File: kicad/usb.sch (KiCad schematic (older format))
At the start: 10 parts, among them J1 USB-C/16p, U2 CH340C, U3 AMS1117-3.3

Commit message: Changelog eingeführt, GND statt GNDD
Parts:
- C1, C2: PriceForQty 500 -> (none)
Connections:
- net labels removed: GNDD
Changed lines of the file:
@@
 F 8 "" H 4100 2400 50  0001 C CNN "PartNr"
 F 9 "0.002141" H 4100 2400 50  0001 C CNN "PriceEUR"
-F 10 "500" H 4100 2400 50  0001 C CNN "PriceForQty"
+F 10 "500
+" H 4100 2400 50  0001 C CNN "PriceForQty"
 F 11 "https://lcsc.com/product-detail/Multilayer-Ceramic-Capacitors-MLCC-SMD-SMT_Walsin-Tech-Corp-0603B104K160CT_C80516.html" H 4100 2400 50  0001 C CNN "Weblink"
 F 12 "C80516" H 4100 2400 50  0001 C CNN "DistOrderNr"
@@
 $EndComp
 $Comp
-L power:GNDD #PWR?
+L power:GND #PWR?
 U 1 1 5F7120DC
 P 4350 2400
@@
 	3350 3000 3400 3000
 $Comp
-L power:GNDD #PWR?
+L power:GND #PWR?
 U 1 1 5F764C96
 P 2900 3000
@@
 F 8 "" H 3400 2400 50  0001 C CNN "PartNr"
 F 9 "0.002141" H 3400 2400 50  0001 C CNN "PriceEUR"
-F 10 "500" H 3400 2400 50  0001 C CNN "PriceForQty"
+F 10 "500
+" H 3400 2400 50  0001 C CNN "PriceForQty"
 F 11 "https://lcsc.com/product-detail/Multilayer-Ceramic-Capacitors-MLCC-SMD-SMT_Walsin-Tech-Corp-0603B104K160CT_C80516.html" H 3400 2400 50  0001 C CNN "Weblink"
 F 12 "C80516" H 3400 2400 50  0001 C CNN "DistOrderNr"
@@
 $EndComp
 $Comp
-L power:GNDD #PWR?
+L power:GND #PWR?
 U 1 1 5F767C48
 P 3150 2400
@@
 $EndComp
 $Comp
-L power:GNDD #PWR?
+L power:GND #PWR?
 U 1 1 60590650
 P 3800 4150
@@
 AR Path="/5F8D661A/60590650" Ref="#PWR012"  Part="1"
 F 0 "#PWR012" H 3800 3900 50  0001 C CNN
-F 1 "GNDD" H 3804 3995 50  0000 C CNN
+F 1 "GND" H 3804 3995 50  0000 C CNN
 F 2 "" H 3800 4150 50  0001 C CNN
 F 3 "" H 3800 4150 50  0001 C CNN
@@
 $EndComp
 $Comp
-L power:GNDD #PWR?
+L power:GND #PWR?
 U 1 1 605914DB
 P 1350 4200
@@
 AR Path="/5F8D661A/605914DB" Ref="#PWR07"  Part="1"
 F 0 "#PWR07" H 1350 3950 50  0001 C CNN
-F 1 "GNDD" H 1354 4045 50  0000 C CNN
+F 1 "GND" H 1354 4045 50  0000 C CNN
 F 2 "" H 1350 4200 50  0001 C CNN
 F 3 "" H 1350 4200 50  0001 C CNN
@@
 $EndComp
 $Comp
-L power:GNDD #PWR?
+L power:GND #PWR?
 U 1 1 60591BD5
 P 1650 4200
@@
 AR Path="/5F8D661A/60591BD5" Ref="#PWR08"  Part="1"
 F 0 "#PWR08" H 1650 3950 50  0001 C CNN
-F 1 "GNDD" H 1654 4045 50  0000 C CNN
+F 1 "GND" H 1654 4045 50  0000 C CNN
 F 2 "" H 1650 4200 50  0001 C CNN
 F 3 "" H 1650 4200 50  0001 C CNN
@@
 $EndComp
 $Comp
-L power:GNDD #PWR?
+L power:GND #PWR?
 U 1 1 605932E8
 P 6300 2350
@@
 AR Path="/5F8D661A/605932E8" Ref="#PWR014"  Part="1"
 F 0 "#PWR014" H 6300 2100 50  0001 C CNN
-F 1 "GNDD" H 6304 2195 50  0000 C CNN
+F 1 "GND" H 6304 2195 50  0000 C CNN
 F 2 "" H 6300 2350 50  0001 C CNN
 F 3 "" H 6300 2350 50  0001 C CNN
@@
 $EndComp
 $Comp
-L power:GNDD #PWR?
+L power:GND #PWR?
 U 1 1 605939B6
 P 6850 2350
@@
 AR Path="/5F8D661A/605939B6" Ref="#PWR015"  Part="1"
 F 0 "#PWR015" H 6850 2100 50  0001 C CNN
-F 1 "GNDD" H 6854 2195 50  0000 C CNN
+F 1 "GND" H 6854 2195 50  0000 C CNN
 F 2 "" H 6850 2350 50  0001 C CNN
 F 3 "" H 6850 2350 50  0001 C CNN
@@
 $EndComp
 $Comp
-L power:GNDD #PWR?
+L power:GND #PWR?
 U 1 1 60594161
 P 7250 2350
@@
 AR Path="/5F8D661A/60594161" Ref="#PWR016"  Part="1"
 F 0 "#PWR016" H 7250 2100 50  0001 C CNN
-F 1 "GNDD" H 7254 2195 50  0000 C CNN
+F 1 "GND" H 7254 2195 50  0000 C CNN
 F 2 "" H 7250 2350 50  0001 C CNN
 F 3 "" H 7250 2350 50  0001 C CNN

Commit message: usb.sch Datei war gebrochen, wurde gefixt
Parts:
- C1, C2: PriceForQty (none) -> 500
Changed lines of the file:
@@
 F 8 "" H 4100 2400 50  0001 C CNN "PartNr"
 F 9 "0.002141" H 4100 2400 50  0001 C CNN "PriceEUR"
-F 10 "500
-" H 4100 2400 50  0001 C CNN "PriceForQty"
+F 10 "500" H 4100 2400 50  0001 C CNN "PriceForQty"
 F 11 "https://lcsc.com/product-detail/Multilayer-Ceramic-Capacitors-MLCC-SMD-SMT_Walsin-Tech-Corp-0603B104K160CT_C80516.html" H 4100 2400 50  0001 C CNN "Weblink"
 F 12 "C80516" H 4100 2400 50  0001 C CNN "DistOrderNr"
@@
 F 8 "" H 3400 2400 50  0001 C CNN "PartNr"
 F 9 "0.002141" H 3400 2400 50  0001 C CNN "PriceEUR"
-F 10 "500
-" H 3400 2400 50  0001 C CNN "PriceForQty"
+F 10 "500" H 3400 2400 50  0001 C CNN "PriceForQty"
 F 11 "https://lcsc.com/product-detail/Multilayer-Ceramic-Capacitors-MLCC-SMD-SMT_Walsin-Tech-Corp-0603B104K160CT_C80516.html" H 3400 2400 50  0001 C CNN "Weblink"
 F 12 "C80516" H 3400 2400 50  0001 C CNN "DistOrderNr"

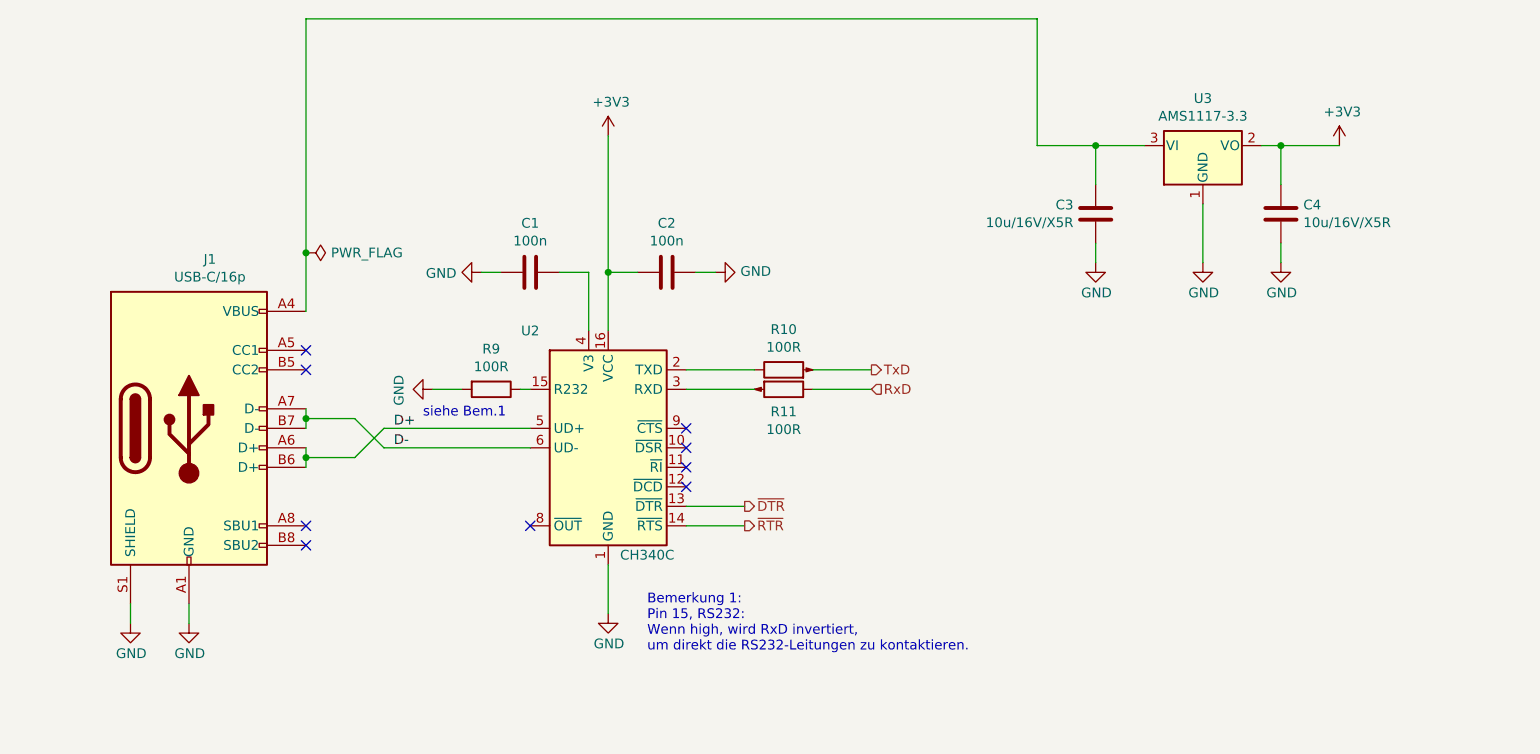
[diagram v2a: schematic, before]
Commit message: Fertiges Layout v0.0.2, 3 Stk bestellt
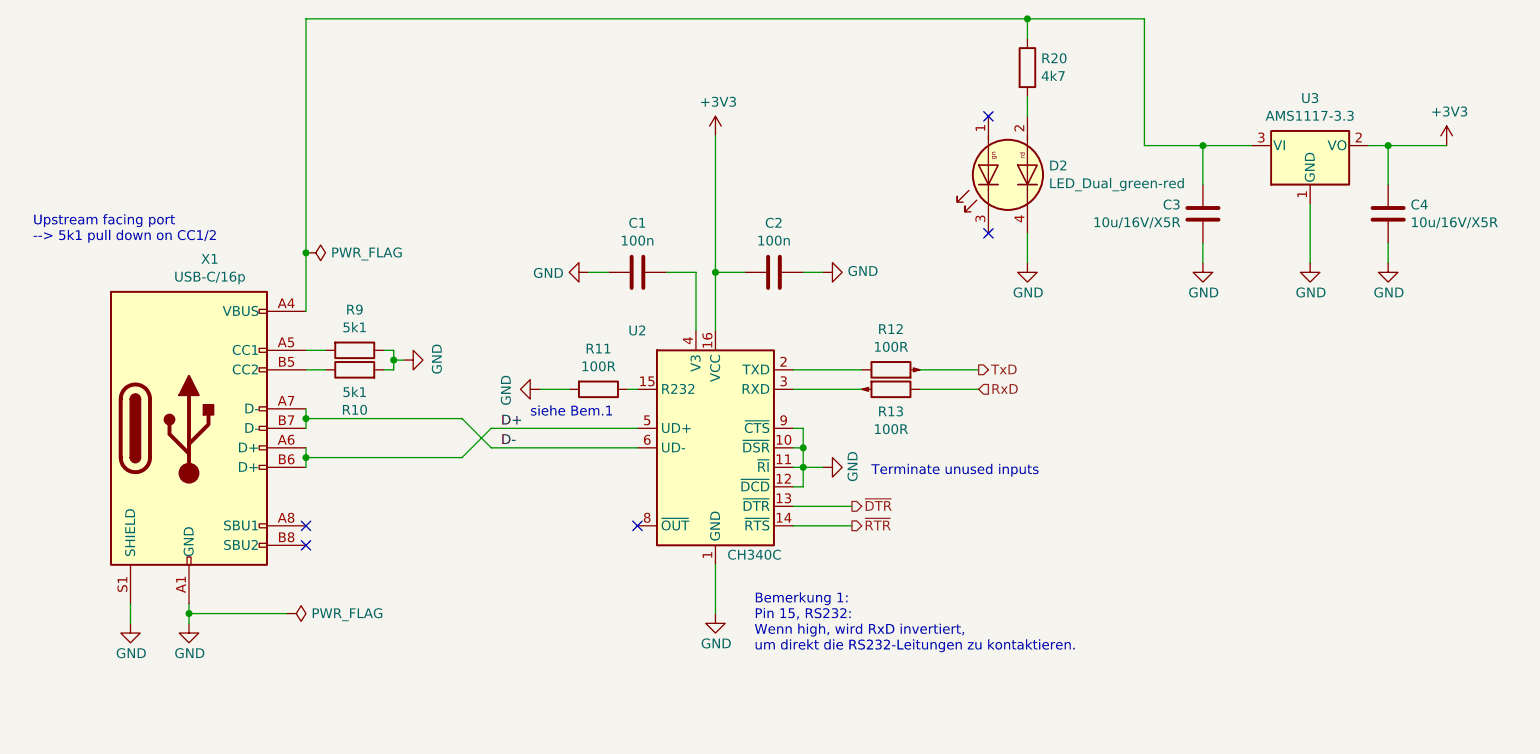
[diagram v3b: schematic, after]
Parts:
- added D2: LED_Dual_green-red, htl_smd:LED_LiteOn_LTST-C195KGJRKT, symbol htl_semiconductors:LED_Dual_green-red
- added R10, R9: 5k1, Resistor_SMD:R_0603_1608Metric, symbol Device:R
- added R20: 4k7, Resistor_SMD:R_0603_1608Metric, symbol Device:R
- renumbered R9 to R11, R10 to R12, R11 to R13, J1 to X1
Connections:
- net GND: now also U2.10 (~DSR), U2.11 (~RI), U2.12 (~DCD), U2.9 (~CTS), D2.4 (K2), R10.2, R9.1
- net at C3.1, U3.3 (VI), X1.A4 (VBUS)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: now also R20.1
- net at X1.A5 (CC1): now also R9.2
- net at X1.B5 (CC2): now also R10.1
- new net: D2.2 (A2), R20.2
- no-connect marks 9 -> 5
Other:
- note added: "Terminate unused inputs"
- note added: "Upstream facing port\n--> 5k1 pull down on CC1/2"
- moved on the sheet: C1, C2, C3, C4, R11, R12, R13, U2, U3

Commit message: BOM fertig eingepflegt
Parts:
- D2: Notes (none) -> Doppel-LED, rot/grün, 2x1608
- R11: DistOrderNr C25201 -> C103204; ManPartNr 0603WAJ0101T5E -> RTT03101JTP; Manufacturer UNI-ROYAL -> RALEC; Notes 100R, 5%, 100mW -> 100Ω ±5% 0.1W ±100ppm/℃; PriceEUR 0.000563 -> 0.0015; PriceForQty 1000 -> 100
- R12, R13: DistOrderNr (none) -> C103204; Distributor (none) -> LCSC; ManPartNr (none) -> RTT03101JTP; Manufacturer (none) -> RALEC; Notes (none) -> 100Ω ±5% 0.1W ±100ppm/℃; PriceEUR (none) -> 0.0015; PriceForQty (none) -> 100
- R20: DistOrderNr (none) -> C103662; Distributor (none) -> LCSC; ManPartNr (none) -> RTT03472JTP; Manufacturer (none) -> RALEC; Notes (none) -> 4.7kΩ ±5% 0.1W ±100ppm/K; PriceEUR (none) -> 0.0015; PriceForQty (none) -> 100
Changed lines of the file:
@@
 F 2 "Resistor_SMD:R_0603_1608Metric" V 3680 3000 50  0001 C CNN
 F 3 "https://datasheet.lcsc.com/szlcsc/Uniroyal-Elec-0603WAJ0101T5E_C25201.pdf" H 3750 3000 50  0001 C CNN
-F 4 "C25201" H 3750 3000 50  0001 C CNN "DistOrderNr"
+F 4 "C103204" H 3750 3000 50  0001 C CNN "DistOrderNr"
 F 5 "LCSC" H 3750 3000 50  0001 C CNN "Distributor"
-F 6 "0603WAJ0101T5E" H 3750 3000 50  0001 C CNN "ManPartNr"
-F 7 "UNI-ROYAL" H 3750 3000 50  0001 C CNN "Manufacturer"
-F 8 "100R, 5%, 100mW" H 3750 3000 50  0001 C CNN "Notes"
-F 9 "0.000563" H 3750 3000 50  0001 C CNN "PriceEUR"
-F 10 "1000" H 3750 3000 50  0001 C CNN "PriceForQty"
+F 6 "RTT03101JTP" H 3750 3000 50  0001 C CNN "ManPartNr"
+F 7 "RALEC" H 3750 3000 50  0001 C CNN "Manufacturer"
+F 8 "100Ω ±5% 0.1W ±100ppm/℃" H 3750 3000 50  0001 C CNN "Notes"
+F 9 "0.0015" H 3750 3000 50  0001 C CNN "PriceEUR"
+F 10 "100" H 3750 3000 50  0001 C CNN "PriceForQty"
 F 11 "https://lcsc.com/product-detail/Chip-Resistor-Surface-Mount_UNI-ROYAL-Uniroyal-Elec-0603WAJ0101T5E_C25201.html" H 3750 3000 50  0001 C CNN "Weblink"
 	1    3750 3000
@@
 F 2 "Resistor_SMD:R_0603_1608Metric" V 5180 2900 50  0001 C CNN
 F 3 "" H 5250 2900 50  0001 C CNN
+F 4 "C103204" H 5250 2900 50  0001 C CNN "DistOrderNr"
+F 5 "LCSC" H 5250 2900 50  0001 C CNN "Distributor"
+F 6 "RTT03101JTP" H 5250 2900 50  0001 C CNN "ManPartNr"
+F 7 "RALEC" H 5250 2900 50  0001 C CNN "Manufacturer"
+F 8 "100Ω ±5% 0.1W ±100ppm/℃" H 5250 2900 50  0001 C CNN "Notes"
+F 9 "0.0015" H 5250 2900 50  0001 C CNN "PriceEUR"
+F 10 "100" H 5250 2900 50  0001 C CNN "PriceForQty"
 	1    5250 2900
 	0    -1   -1   0
@@
 F 2 "Resistor_SMD:R_0603_1608Metric" V 5180 3000 50  0001 C CNN
 F 3 "" H 5250 3000 50  0001 C CNN
+F 4 "C103204" H 5250 3000 50  0001 C CNN "DistOrderNr"
+F 5 "LCSC" H 5250 3000 50  0001 C CNN "Distributor"
+F 6 "RTT03101JTP" H 5250 3000 50  0001 C CNN "ManPartNr"
+F 7 "RALEC" H 5250 3000 50  0001 C CNN "Manufacturer"
+F 8 "100Ω ±5% 0.1W ±100ppm/℃" H 5250 3000 50  0001 C CNN "Notes"
+F 9 "0.0015" H 5250 3000 50  0001 C CNN "PriceEUR"
+F 10 "100" H 5250 3000 50  0001 C CNN "PriceForQty"
 	1    5250 3000
 	0    1    1    0
@@
 F 2 "Resistor_SMD:R_0603_1608Metric" V 5880 1350 50  0001 C CNN
 F 3 "" H 5950 1350 50  0001 C CNN
+F 4 "C103662" H 5950 1350 50  0001 C CNN "DistOrderNr"
+F 5 "LCSC" H 5950 1350 50  0001 C CNN "Distributor"
+F 6 " RTT03472JTP" H 5950 1350 50  0001 C CNN "ManPartNr"
+F 7 "RALEC" H 5950 1350 50  0001 C CNN "Manufacturer"
+F 8 "4.7kΩ ±5% 0.1W ±100ppm/K" H 5950 1350 50  0001 C CNN "Notes"
+F 9 "0.0015" H 5950 1350 50  0001 C CNN "PriceEUR"
+F 10 "100" H 5950 1350 50  0001 C CNN "PriceForQty"
 	1    5950 1350
 	1    0    0    -1
@@
 F 9 "600" H 5850 1900 24  0001 C CNN "PriceForQty"
 F 10 "https://lcsc.com/products/Light-Emitting-Diodes-LED_528.html?q=LTST-C195KGJRKT" H 5850 1900 24  0001 C CNN "Weblink"
+F 11 "Doppel-LED, rot/grün, 2x1608" H 5850 1900 50  0001 C CNN "Notes"
 	1    5850 1900
 	0    -1   1    0

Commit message: BOM für Bestellung bei LCSC nochmals korrigiert
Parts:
- R10, R9: DistOrderNr C25201 -> C150387; ManPartNr 0603WAJ0101T5E -> CR16-512FV; Manufacturer UNI-ROYAL -> HDK(Hokuriku Elec Industry); Notes 100R, 5%, 100mW -> 5k1, 1%, 100mW, 1608
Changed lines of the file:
@@
 F 2 "Resistor_SMD:R_0603_1608Metric" V 2430 2800 50  0001 C CNN
 F 3 "https://datasheet.lcsc.com/szlcsc/Uniroyal-Elec-0603WAJ0101T5E_C25201.pdf" H 2500 2800 50  0001 C CNN
-F 4 "C25201" H 2500 2800 50  0001 C CNN "DistOrderNr"
+F 4 "C150387" H 2500 2800 50  0001 C CNN "DistOrderNr"
 F 5 "LCSC" H 2500 2800 50  0001 C CNN "Distributor"
-F 6 "0603WAJ0101T5E" H 2500 2800 50  0001 C CNN "ManPartNr"
-F 7 "UNI-ROYAL" H 2500 2800 50  0001 C CNN "Manufacturer"
-F 8 "100R, 5%, 100mW" H 2500 2800 50  0001 C CNN "Notes"
+F 6 "CR16-512FV" H 2500 2800 50  0001 C CNN "ManPartNr"
+F 7 "HDK(Hokuriku Elec Industry)" H 2500 2800 50  0001 C CNN "Manufacturer"
+F 8 "5k1, 1%, 100mW, 1608" H 2500 2800 50  0001 C CNN "Notes"
 F 9 "0.000563" H 2500 2800 50  0001 C CNN "PriceEUR"
 F 10 "1000" H 2500 2800 50  0001 C CNN "PriceForQty"
@@
 F 2 "Resistor_SMD:R_0603_1608Metric" V 2430 2900 50  0001 C CNN
 F 3 "https://datasheet.lcsc.com/szlcsc/Uniroyal-Elec-0603WAJ0101T5E_C25201.pdf" H 2500 2900 50  0001 C CNN
-F 4 "C25201" H 2500 2900 50  0001 C CNN "DistOrderNr"
+F 4 "C150387" H 2500 2900 50  0001 C CNN "DistOrderNr"
 F 5 "LCSC" H 2500 2900 50  0001 C CNN "Distributor"
-F 6 "0603WAJ0101T5E" H 2500 2900 50  0001 C CNN "ManPartNr"
-F 7 "UNI-ROYAL" H 2500 2900 50  0001 C CNN "Manufacturer"
-F 8 "100R, 5%, 100mW" H 2500 2900 50  0001 C CNN "Notes"
+F 6 "CR16-512FV" H 2500 2900 50  0001 C CNN "ManPartNr"
+F 7 "HDK(Hokuriku Elec Industry)" H 2500 2900 50  0001 C CNN "Manufacturer"
+F 8 "5k1, 1%, 100mW, 1608" H 2500 2900 50  0001 C CNN "Notes"
 F 9 "0.000563" H 2500 2900 50  0001 C CNN "PriceEUR"
 F 10 "1000" H 2500 2900 50  0001 C CNN "PriceForQty"
